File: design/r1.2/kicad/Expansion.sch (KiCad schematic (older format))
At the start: 29 parts, among them IC1 MC68010P10, IC4 MC68901P, IC6 74174N, IC9 74LS01N, J1 PWR, J3 Conn_02x32_Odd_Even, J4 Conn_01x06, J5 GPIO-PANEL

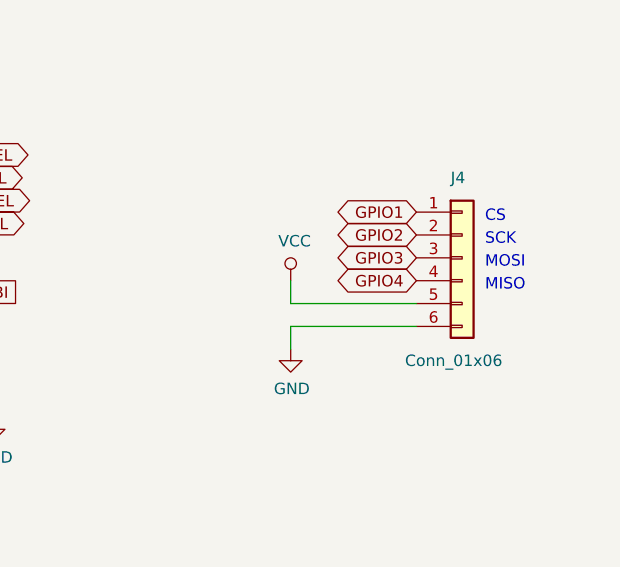
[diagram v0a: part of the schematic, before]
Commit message: Revert "Merge pull request #181 from rosco-m68k/feature/board-1.22"
This reverts commit 67e3259ef153c8a657db8d826cd60eea2d9b52e3, reversing
changes made to 43bb90592578d0b0c5d0a3f828a55b4324962c1a.
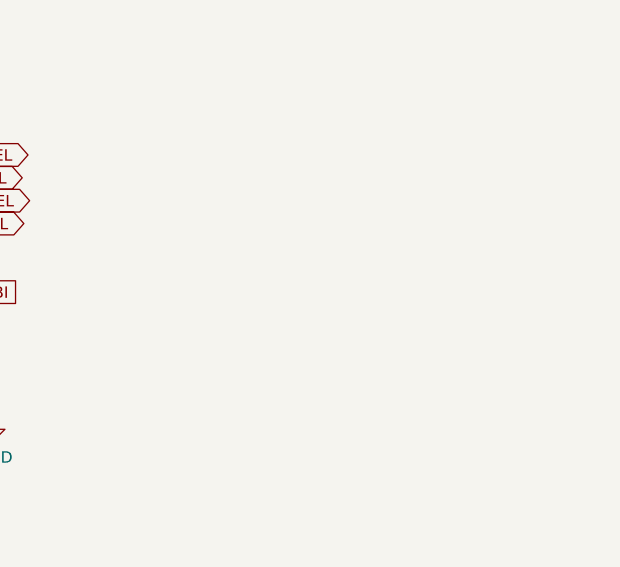
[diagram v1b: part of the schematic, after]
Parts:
- removed J4: Conn_01x06, rosco_m68k:1X06, symbol Connector_Generic:Conn_01x06
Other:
- note removed: "CS"
- note removed: "MISO"
- note removed: "MOSI"
- note removed: "SCK"
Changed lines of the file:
@@
 Sheet 4 4
 Title "EXPANSION AND MECHANICAL"
-Date "2021-03-05"
-Rev "1.22"
-Comp "The Really Old-School Company Limited"
+Date "2020-05-26"
+Rev "1.2"
+Comp ""
 Comment1 "OSHWA UK000006 (https://certification.oshwa.org/uk000006.html)"
 Comment2 "See https://github.com/roscopeco/rosco_m68k/blob/master/LICENCE.hardware.txt"
 Comment3 "Open Source Hardware licenced under CERN Open Hardware Licence"
-Comment4 "Copyright 2019-2021 Ross Bamford and Contributors"
+Comment4 "Copyright 2019-2020 Ross Bamford and Contributors"
 $EndDescr
 Wire Wire Line
@@
 Wire Wire Line
 	10950 7400 10950 7850
-$Comp
-L Connector_Generic:Conn_01x06 J?
-U 1 1 60465FFE
-P 13000 7150
-AR Path="/5E53B4B8/60465FFE" Ref="J?"  Part="1"
-AR Path="/5E53BC83/60465FFE" Ref="J4"  Part="1"
-F 0 "J4" H 12950 7500 50  0000 L CNN
-F 1 "Conn_01x06" H 12750 6700 50  0000 L CNN
-F 2 "rosco_m68k:1X06" H 13000 7150 50  0001 C CNN
-F 3 "~" H 13000 7150 50  0001 C CNN
-	1    13000 7150
-	1    0    0    -1
-$EndComp
-Text GLabel 12800 6950 0    50   BiDi ~ 0
-GPIO1
-Text Notes 13100 7000 0    50   ~ 0
-CS
-Text Notes 13100 7100 0    50   ~ 0
-SCK
-Text GLabel 12800 7050 0    50   BiDi ~ 0
-GPIO2
-Text GLabel 12800 7150 0    50   BiDi ~ 0
-GPIO3
-Text GLabel 12800 7250 0    50   BiDi ~ 0
-GPIO4
-Text Notes 13100 7200 0    50   ~ 0
-MOSI
-Text Notes 13100 7300 0    50   ~ 0
-MISO
-$Comp
-L power:VCC #PWR0129
-U 1 1 604703CB
-P 12250 7250
-F 0 "#PWR0129" H 12250 7100 50  0001 C CNN
-F 1 "VCC" H 12267 7423 50  0000 C CNN
-F 2 "" H 12250 7250 50  0001 C CNN
-F 3 "" H 12250 7250 50  0001 C CNN
-	1    12250 7250
-	1    0    0    -1
-$EndComp
-$Comp
-L power:GND #PWR0130
-U 1 1 60470D8A
-P 12250 7550
-F 0 "#PWR0130" H 12250 7300 50  0001 C CNN
-F 1 "GND" H 12255 7377 50  0000 C CNN
-F 2 "" H 12250 7550 50  0001 C CNN
-F 3 "" H 12250 7550 50  0001 C CNN
-	1    12250 7550
-	1    0    0    -1
-$EndComp
-Wire Wire Line
-	12800 7350 12250 7350
-Wire Wire Line
-	12250 7350 12250 7250
-Wire Wire Line
-	12800 7450 12250 7450
-Wire Wire Line
-	12250 7450 12250 7550
 Wire Bus Line
 	11150 4100 11150 5700
